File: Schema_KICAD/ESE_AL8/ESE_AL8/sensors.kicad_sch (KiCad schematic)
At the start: 18 parts, among them J1 CB1, J2 CB2, J3 LIDAR, J4 Moteur1, J5 Moteur2, SW1 SW_c/s, U1 ADXL343

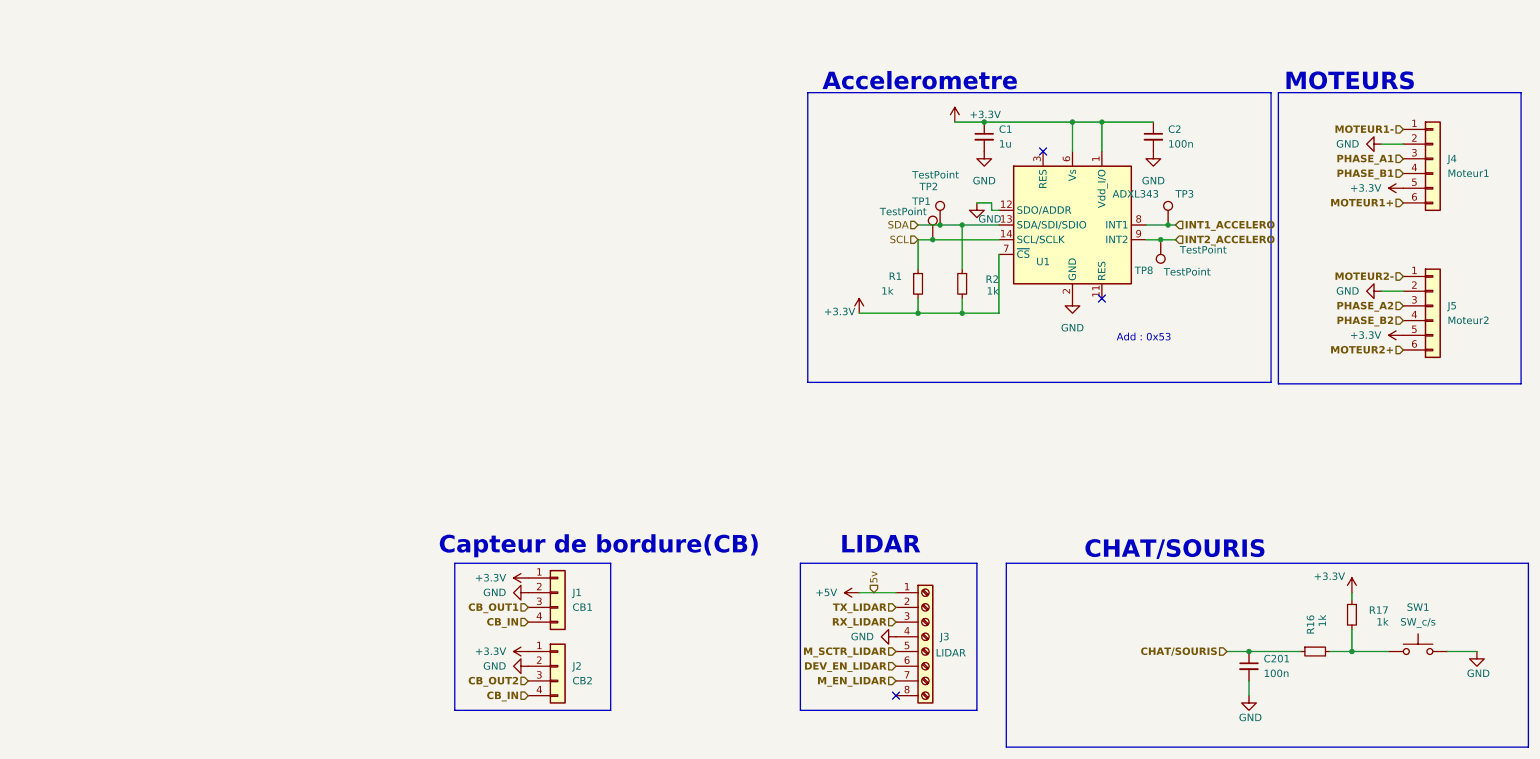
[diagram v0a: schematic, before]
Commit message: le bon ioc
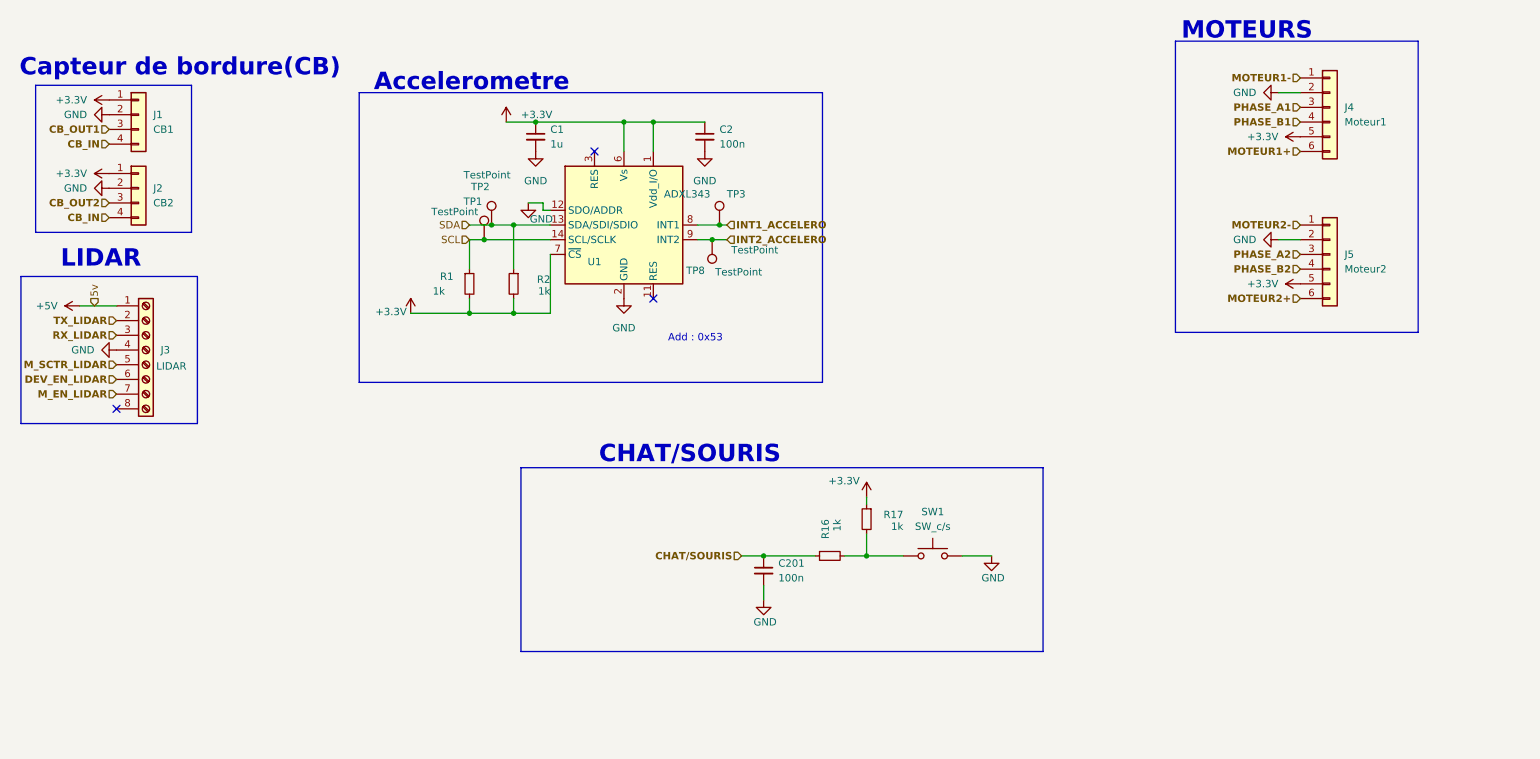
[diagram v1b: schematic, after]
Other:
- moved on the sheet: C1, C2, C201, J1, J2, J3, J4, J5, R1, R16, R17, R2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
